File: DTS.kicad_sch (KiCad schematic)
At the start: 5 parts, among them J4 Conn_01x06_Pin, J5 Conn_01x01_Pin, J6 Conn_01x02_Pin, J7 Conn_01x06_Pin, U23 4069

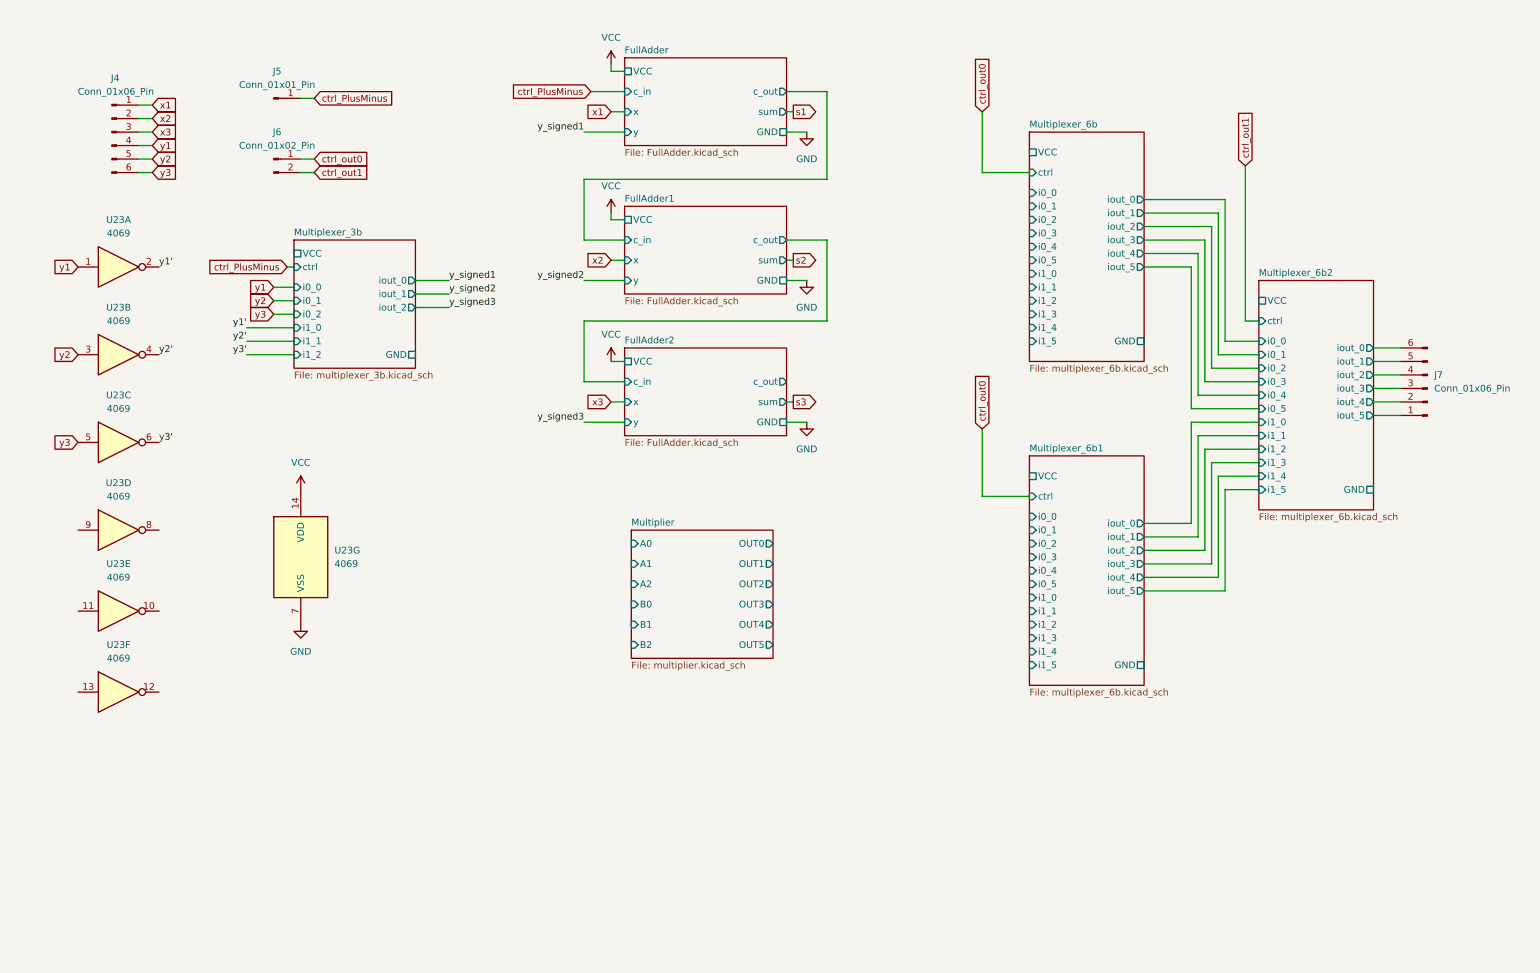
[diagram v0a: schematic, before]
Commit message: Add files via upload
Waiting for approval
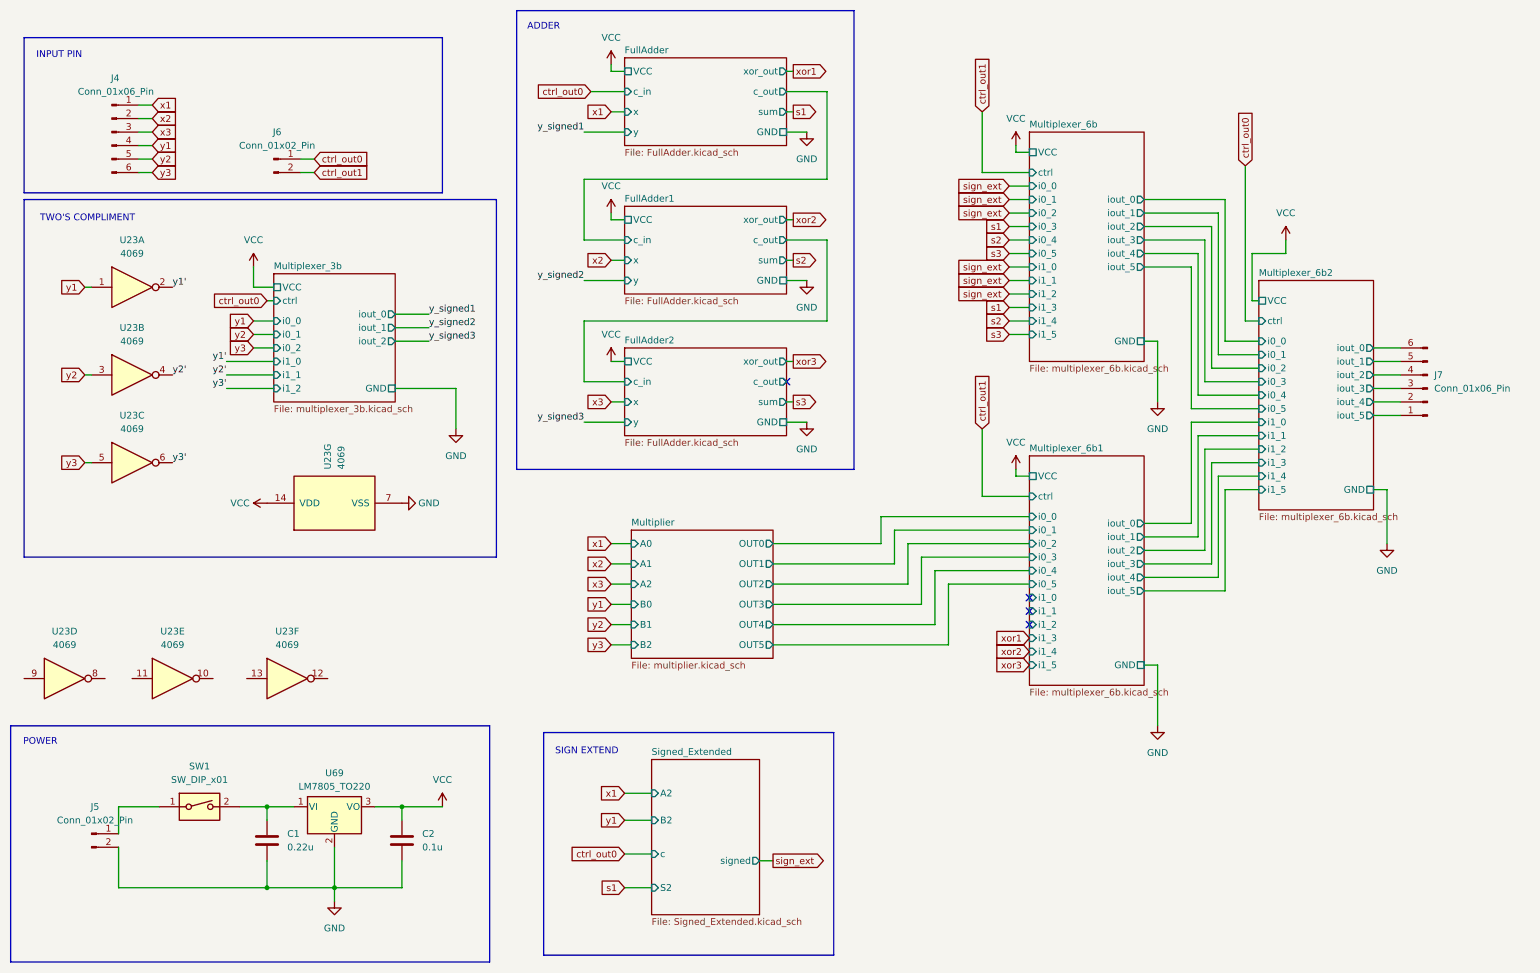
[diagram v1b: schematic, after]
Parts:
- removed J5: Conn_01x01_Pin, symbol Connector:Conn_01x01_Pin
- added C1: 0.22u, symbol Device:C
- added C2: 0.1u, symbol Device:C
- added J5: Conn_01x02_Pin, symbol Connector:Conn_01x02_Pin
- added SW1: SW_DIP_x01, symbol Switch:SW_DIP_x01
- added U69: LM7805_TO220, Package_TO_SOT_THT:TO-220-3_Vertical, symbol Regulator_Linear:LM7805_TO220
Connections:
- net GND: now also C1.2, C2.2, J5.2 (Pin_2), U69.2 (GND)
- net VCC: now also C2.1, U69.3 (VO)
- new net: J5.1 (Pin_1), SW1.1
- new net: C1.1, SW1.2, U69.1 (VI)
- no-connect marks 0 -> 4
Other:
- added sheet Signed_Extended (Signed_Extended.kicad_sch)
- sheet FullAdder ports: added xor_out; removed none
- sheet FullAdder1 ports: added xor_out; removed none
- sheet FullAdder2 ports: added xor_out; removed none
- note added: "ADDER"
- note added: "INPUT PIN"
- note added: "POWER"
- note added: "SIGN EXTEND"
- note added: "TWO'S COMPLIMENT"
- moved on the sheet: U23A, U23B, U23C, U23D, U23E, U23F, U23G
